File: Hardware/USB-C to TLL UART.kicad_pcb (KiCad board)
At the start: 2 copper layers, 26 x 30 mm, 13 parts, among them IC1 74LVC1G08SE-7, J1 Conn_01x06_Female, P1 USB_C_Plug_USB2.0, U1 CH340C, U2 AP2112K-3.3

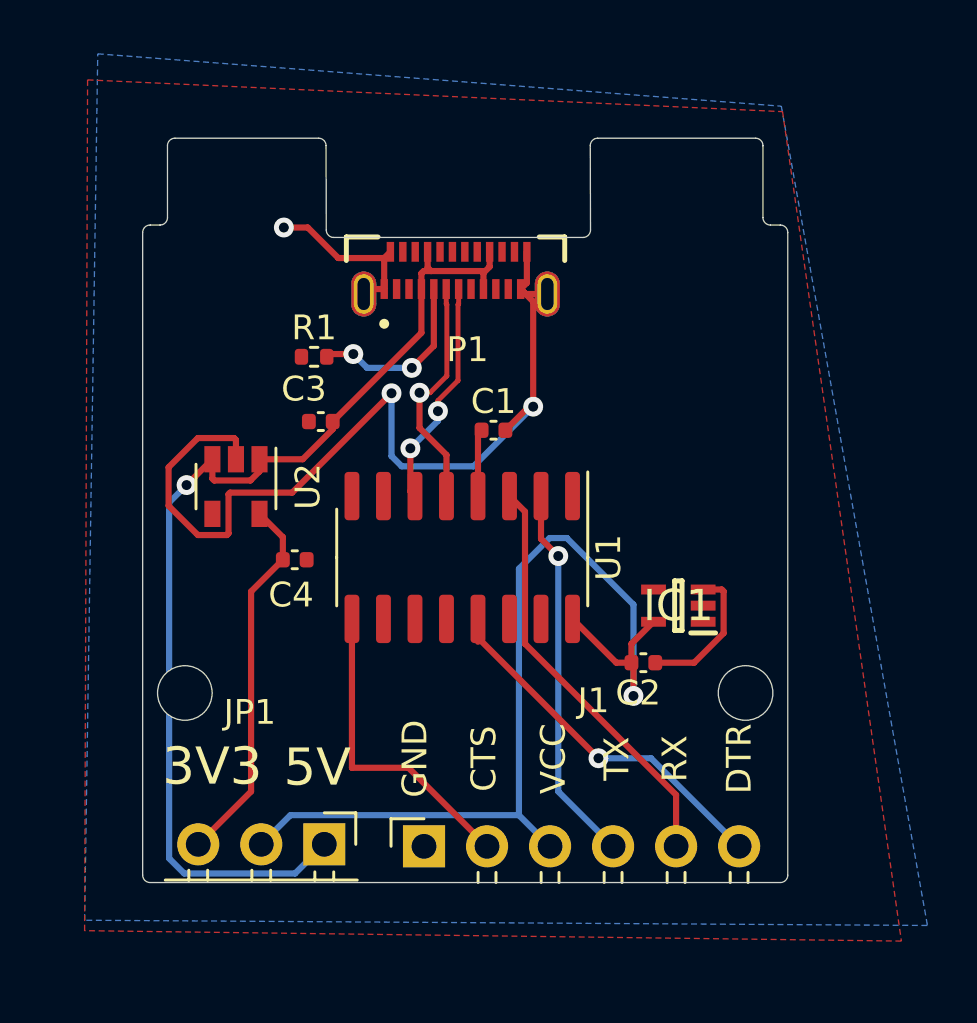
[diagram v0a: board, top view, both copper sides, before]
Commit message: Updated Files
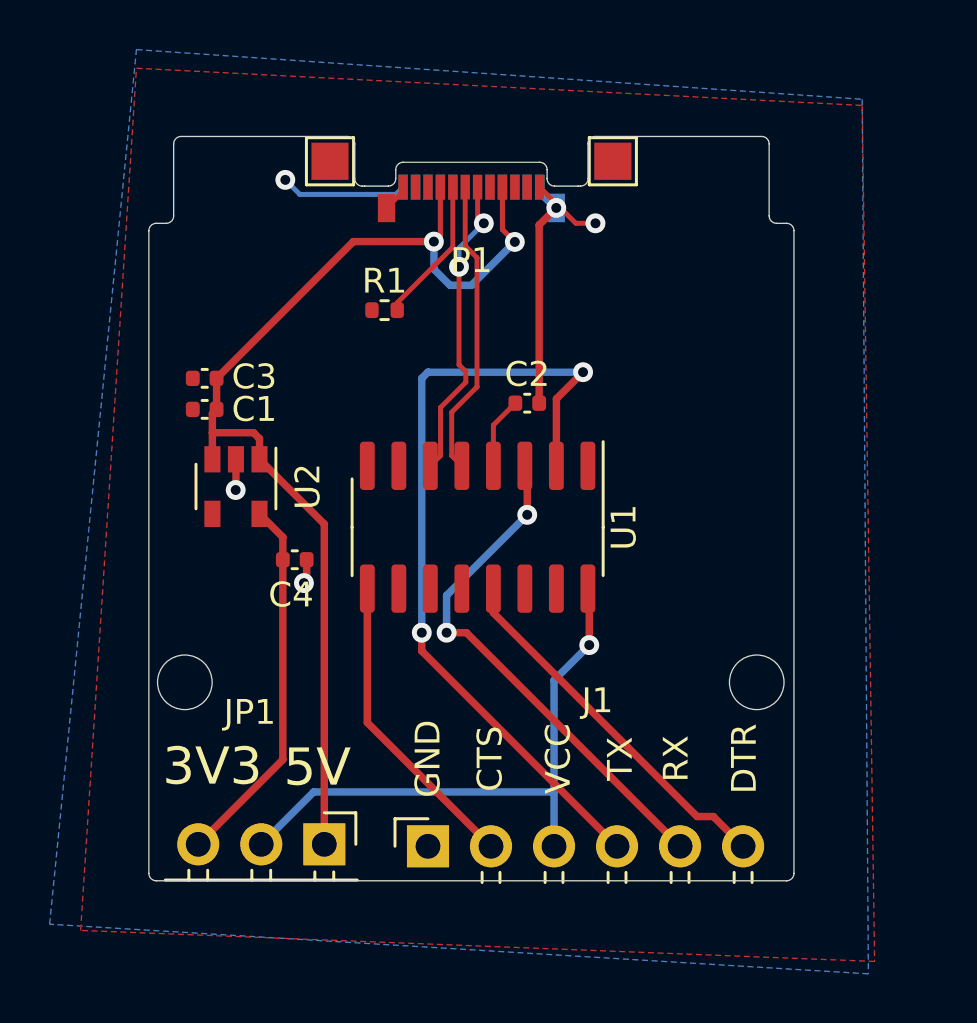
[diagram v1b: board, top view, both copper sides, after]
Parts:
- removed IC1: 74LVC1G08SE-7, SamacSys_Parts:SOT65P210X110-5N
- added TP1: TestPoint, TestPoint:TestPoint_Pad_1.5x1.5mm, F.Cu at (137.6, 89.0)
- added TP3: TestPoint, TestPoint:TestPoint_Pad_1.5x1.5mm, F.Cu at (148.9, 89.0)
- C1: value 10nF -> 0.1uF
- C2: value 100nF -> 10nF
- P1: footprint SnapEDA Library:GCT_USB4155-03-C_REVA -> Expansion_Card:USB_C_Plug_Molex_105444
- moved C1 11.8 mm to (132.5, 97.8), turned to 180 degrees
- moved C2 11.5 mm to (145.5, 98.8)
- moved C3 4.71 mm to (132.5, 99.0)
- moved P1 3.46 mm to (143.2, 90.0), turned to 0 degrees
- moved R1 3.41 mm to (139.8, 95.0)
- moved U1 1.37 mm to (143.5, 103.8)
- moved H2 0.62 mm to (154.8, 110.0)
- moved H1 0.43 mm to (131.7, 110.0)
- moved J1 0.16 mm to (141.5, 116.6)
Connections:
- C1 pad 1: Net-(C1-Pad1) -> 5V
- C2 pad 1: VCC -> Net-(C2-Pad1)
- U1 pad 1: Earth -> Net-(U1-Pad1)
- U1 pad 4: Net-(C1-Pad1) -> Net-(C2-Pad1)
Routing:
- net Earth: track 49.8 -> 21.6 mm, vias 3 -> 5
- net TXO: track 15.6 -> 33.0 mm, vias 1 -> 2
- net VCC: track 39.0 -> 23.7 mm
- net 5V: track 43.4 -> 48.6 mm, vias 1 -> 2
- net RXI: track 16.9 -> 21.1 mm, vias 0 -> 2
- net D-: track 9.23 -> 12.5 mm
- net Net-(C2-Pad1): track 0.00 -> 2.89 mm
- net Net-(C1-Pad1): track 2.72 -> 0.00 mm
- net D+: track 9.51 -> 12.0 mm, vias 1 -> 0
- net Net-(P1-PadA5): track 7.25 -> 5.89 mm, vias 2 -> 0
- net DTR: track 15.7 -> 14.9 mm, vias 1 -> 0
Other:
- outline, holes or cut-outs redrawn
